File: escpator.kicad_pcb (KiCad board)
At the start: 4 copper layers, 45.7 x 15 mm, 38 parts, among them J1 Conn_01x04_Pin, J2 Conn_02x05_Odd_Even, J3 Conn_01x05, U1 STM32F103CBTx, U4 MCP1700x-330xxTT, Y1 Crystal_GND24

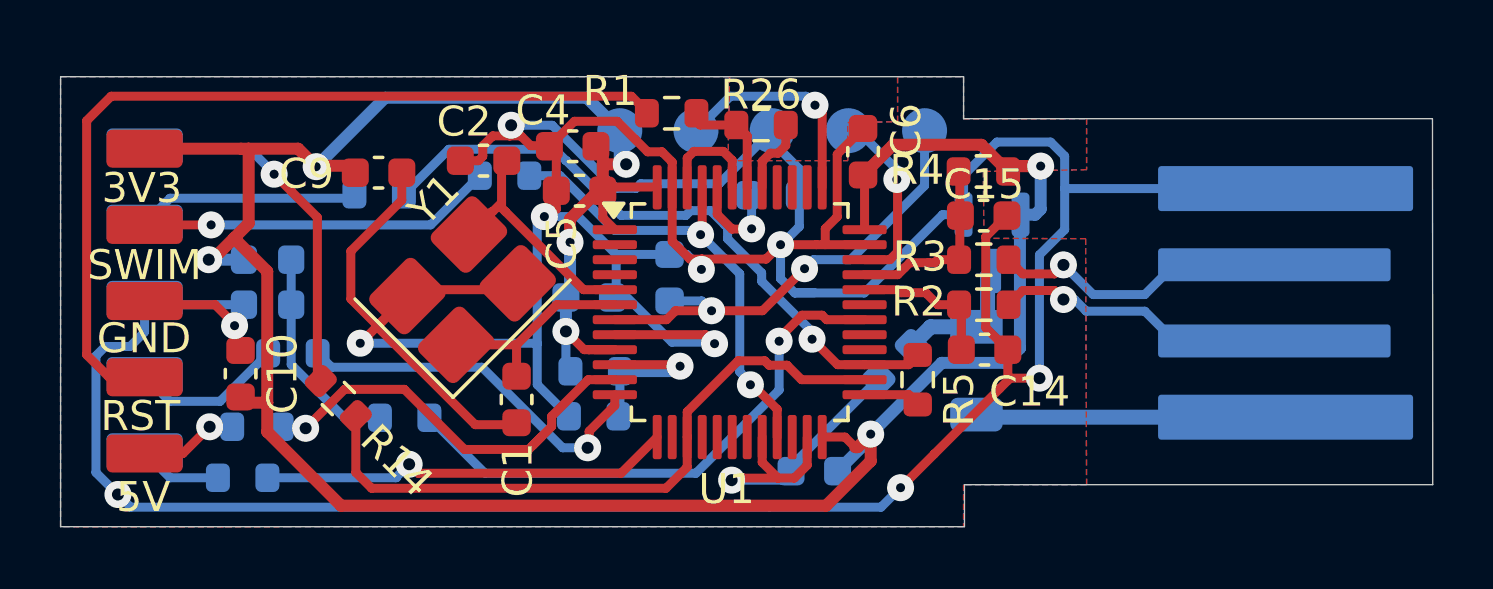
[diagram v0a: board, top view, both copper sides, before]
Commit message: c
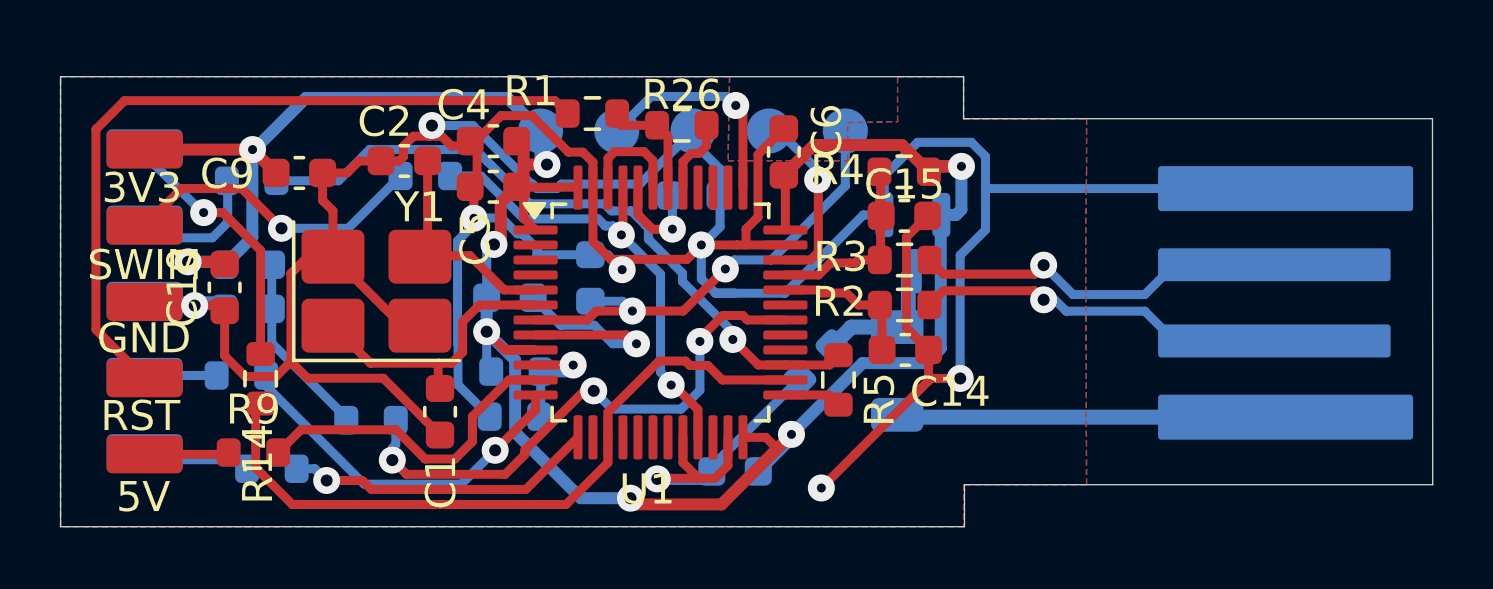
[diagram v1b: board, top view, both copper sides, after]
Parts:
- R9: moved to F.Cu
- moved R13 4.27 mm to (30.8, 33.1)
- moved C10 2.92 mm to (29.9, 36.7), turned to -90 degrees
- moved C5 2.87 mm to (38.9, 33.3)
- moved Y1 2.87 mm to (35.0, 36.8), turned to 0 degrees
- moved R14 2.67 mm to (31.1, 39.7), turned to 90 degrees
- moved C4 2.65 mm to (38.9, 31.8)
- moved C15 2.64 mm to (52.6, 34.3)
- moved R2 2.64 mm to (52.6, 37.2)
- moved R3 2.64 mm to (52.6, 35.7)
- moved R24 2.64 mm to (39.6, 41.0)
- moved C11 2.64 mm to (42.1, 36.3)
- moved C14 2.64 mm to (52.6, 38.7)
- moved C2 2.64 mm to (35.9, 32.4)
- moved C3 2.64 mm to (49.6, 39.2)
- moved C6 2.64 mm to (48.5, 32.1)
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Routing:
- net Earth: track 185.9 -> 149.5 mm, vias 11 -> 9
- net +3V3: track 96.6 -> 78.5 mm, vias 7 -> 8
- net Net-(J2-Pin_2): track 13.1 -> 8.86 mm
- net Net-(J2-Pin_4): track 8.84 -> 4.57 mm
- net Net-(J2-Pin_7): track 29.4 -> 25.3 mm
- net /STLINK_RX: track 13.8 -> 10.4 mm
- net Net-(J1-Pin_1): track 9.97 -> 13.1 mm
- net /Pin_navic: track 14.0 -> 10.9 mm, vias 1 -> 0
- net /OSC_OUT: track 6.93 -> 9.65 mm
- net Net-(J2-Pin_8): track 5.13 -> 2.43 mm
- net /D+: track 10.0 -> 12.6 mm
- net /D-: track 9.75 -> 12.4 mm
- net /AIN1: track 5.97 -> 4.12 mm
- net /OSC_IN?: track 8.90 -> 7.20 mm
- net Net-(J2-Pin_3): track 11.9 -> 10.3 mm
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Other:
- copper layers 4 -> 2
